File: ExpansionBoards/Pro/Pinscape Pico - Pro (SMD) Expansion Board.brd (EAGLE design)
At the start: 170.6 x 108 mm, 179 parts, among them IC1 UCC27523D, IC10 UCC27523D, IC11 UCC27523D, IC12 UCC27523D, IC13 UCC27523D, IC14 UCC27523D, IC15 TLC59116FIRHBR, IC16 TLC59116FIRHBR, IC17 TLC59116FIRHBR, IC18 TLC59116FIRHBR, IC19 ULN2803ADWR, IC2 UCC27523D, IC20 ULN2803ADWR, IC21 ULN2803ADWR, IC22 ULN2803ADWR, IC23 ULN2803ADWR, IC24 PCA9555APW,118, IC25 PCA9555APW,118, IC26 LIS3DHTR, IC27 SN74LVC1G175DCKR, IC28 APX809S-29SA-7, IC29 LTV-827S, IC3 UCC27523D, IC30 ADS1115IDGSR, IC31 TLV75733PDBVR, IC33 RV-3032-C7, IC4 UCC27523D, IC5 UCC27523D, IC6 UCC27523D, IC7 UCC27523D, IC8 UCC27523D, IC9 UCC27523D, J1 640445-6, J10 1-640456-0, J11 1-640456-0, J12 1-640456-0, J13 640445-5, J14 640445-9, J15 640445-9, J16 640445-9, J18 BM03B-SRSS-TB(LF)(SN), J2 30316-6002HB, J3 1-640456-0, J4 640456-9, J5 640456-9, J6 640454-2, J7 215079-4, J8 30308-6002HB, J9 1-640456-0, Q1 BUK7K89-100EX, Q10 BUK7K89-100EX, Q11 BUK7K89-100EX, Q12 BUK7K89-100EX, Q13 BUK7K89-100EX, Q14 BUK7K89-100EX, Q15 UMA5NTR, Q16 UMA5NTR, Q17 UMA5NTR, Q18 UMA5NTR, Q19 UMA5NTR, Q2 BUK7K89-100EX, Q20 UMA5NTR, Q21 UMA5NTR, Q22 UMA5NTR, Q23 UMA5NTR, Q24 UMA5NTR, Q25 UMA5NTR, Q26 UMA5NTR, Q29 DMG2302UK-7, Q3 BUK7K89-100EX, Q4 BUK7K89-100EX, Q5 BUK7K89-100EX, Q6 BUK7K89-100EX, Q7 BUK7K89-100EX, Q8 BUK7K89-100EX, Q9 BUK7K89-100EX, SW1 TS-1187A-B-A-B, U1 BAT-HLD-001-THM

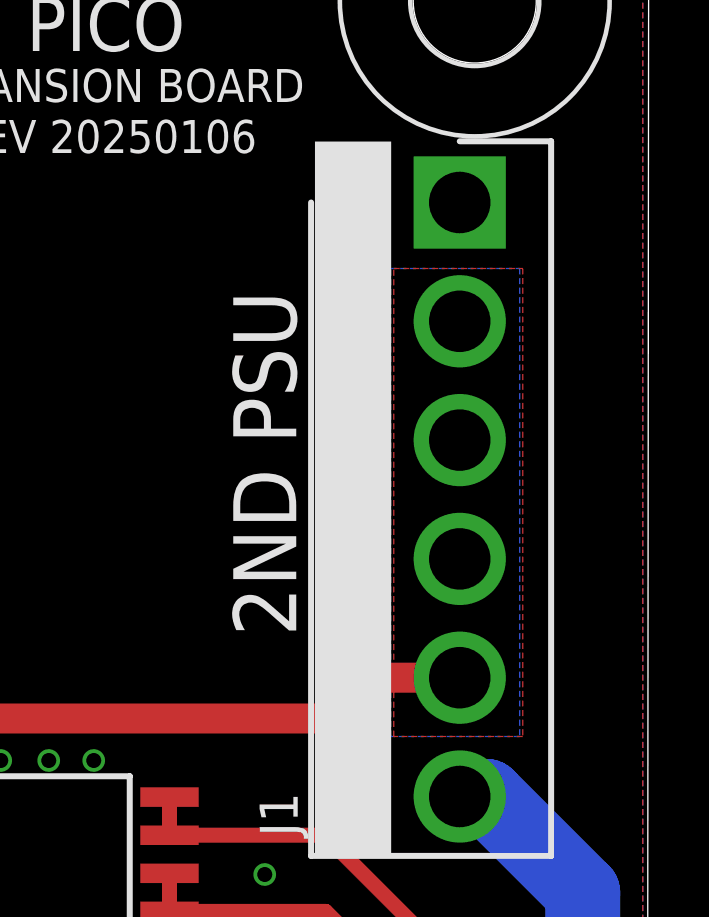
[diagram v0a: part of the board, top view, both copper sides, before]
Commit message: add logo image
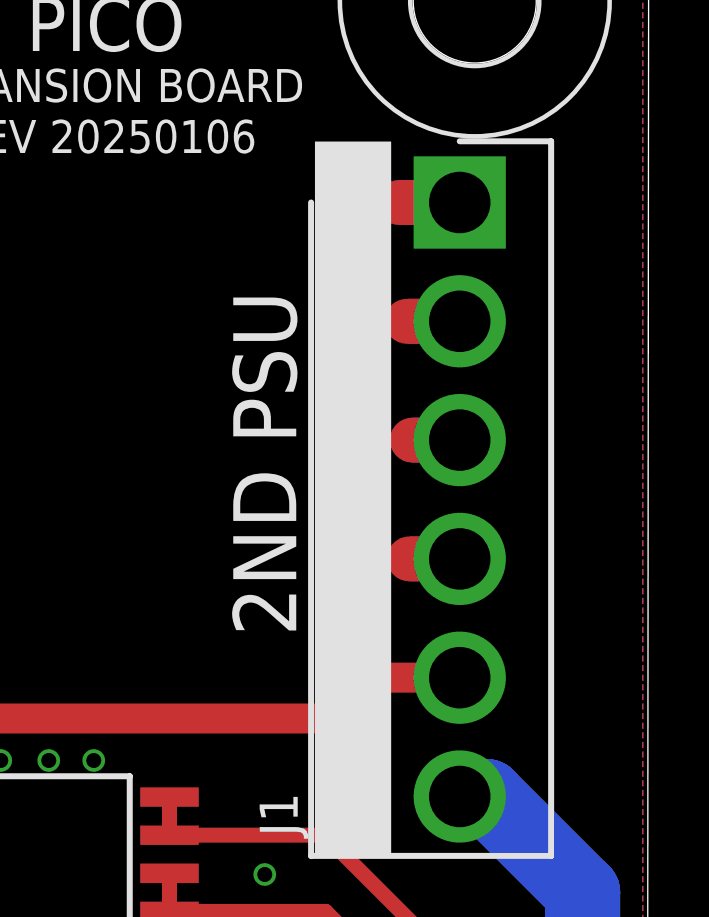
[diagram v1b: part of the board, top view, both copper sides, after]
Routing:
- net GND: track 103.0 -> 116.7 mm
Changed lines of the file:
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@@
 <via x="138" y="22.9" extent="1-16" drill="0.5"/>
 <via x="138.7" y="9.4" extent="1-16" drill="0.5"/>
-<polygon width="0.2" layer="1" thermals="no">
-<vertex x="155.1" y="92.9"/>
-<vertex x="159.4" y="92.9"/>
-<vertex x="159.4" y="77.3"/>
-<vertex x="155.1" y="77.3"/>
-</polygon>
-<polygon width="0.2" layer="16" thermals="no">
-<vertex x="155" y="92.9"/>
-<vertex x="159.3" y="92.9"/>
-<vertex x="159.3" y="77.3"/>
-<vertex x="155" y="77.3"/>
-</polygon>
 <contactref element="J1" pad="1"/>
+<wire x1="157.3" y1="91.14" x2="155.64" y2="91.14" width="1.5" layer="16"/>
+<wire x1="157.3" y1="87.18" x2="155.78" y2="87.18" width="1.5" layer="16"/>
+<wire x1="157.3" y1="83.22" x2="155.72" y2="83.22" width="1.5" layer="16"/>
+<wire x1="157.3" y1="95.1" x2="155.3" y2="95.1" width="1.5" layer="16"/>
+<wire x1="157.3" y1="95.1" x2="155.3" y2="95.1" width="1.5" layer="1"/>
+<wire x1="157.3" y1="91.14" x2="155.54" y2="91.14" width="1.5" layer="1"/>
+<wire x1="157.3" y1="87.18" x2="155.72" y2="87.18" width="1.5" layer="1"/>
+<wire x1="157.3" y1="83.22" x2="155.62" y2="83.22" width="1.5" layer="1"/>
 </signal>
 <signal name="5V">
